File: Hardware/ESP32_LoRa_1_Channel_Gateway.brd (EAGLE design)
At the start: 25.4 x 45.7 mm, 84 parts, among them J3 USB, J4 QWIIC, J6 U.FL, Q1 MBT3904DW1T1, U1 3.3V, U2 CH340C, U3 ESP-WROOM-32NARROW, U4 RFM96W

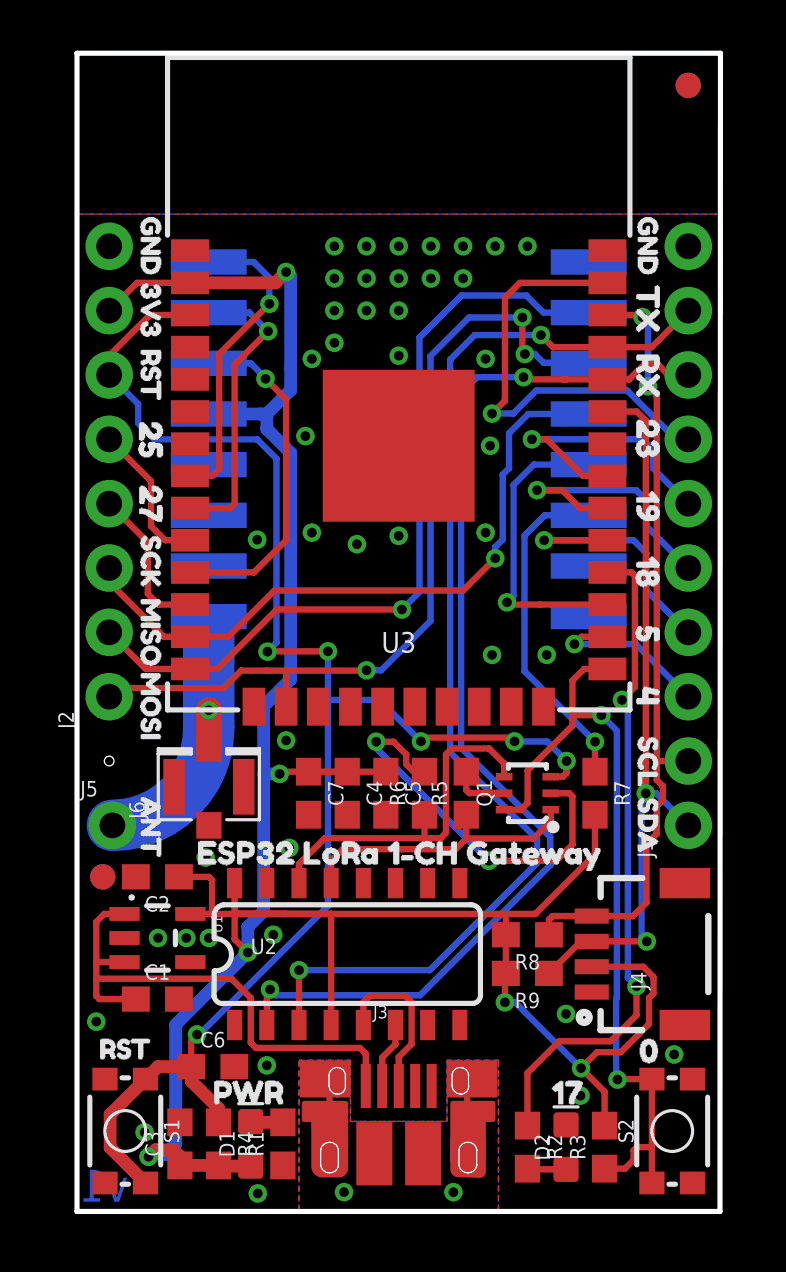
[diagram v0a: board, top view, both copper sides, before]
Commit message: Made changes from REDS review pt 1
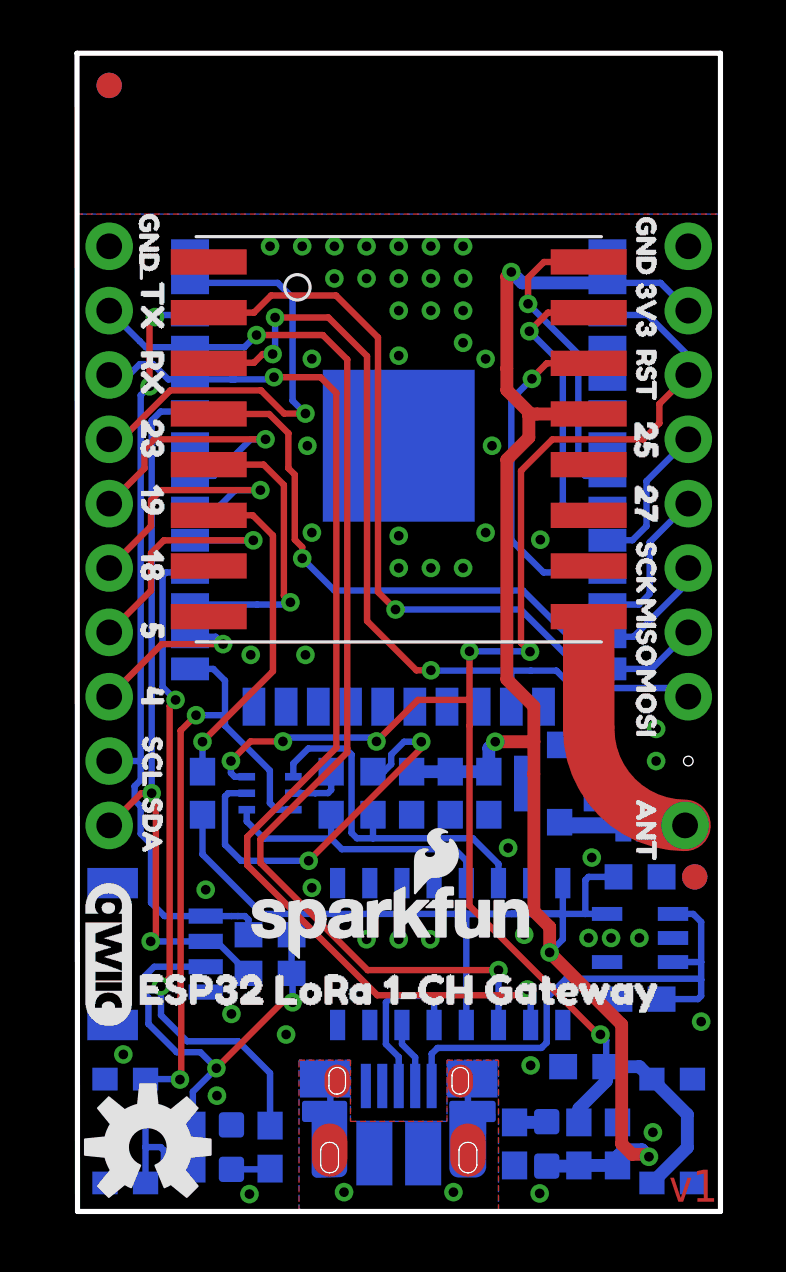
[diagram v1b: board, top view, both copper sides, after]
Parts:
- added JP1: JUMPER-SMT_2_NO_SILK, SparkFun-Jumpers:SMT-JUMPER_2_NO_SILK
- moved U$20 25.0 mm to (25.2, 6.41), flipped to the bottom
- moved FD3 23.4 mm to (24.4, 13.2), flipped to the bottom
- moved FD4 23.4 mm to (24.4, 13.2), flipped to the top
- moved U$9 23.0 mm to (25.9, 16.9), flipped to the bottom, turned to 0 degrees
- moved FD1 22.9 mm to (1.27, 44.5), flipped to the bottom
- moved FD2 22.9 mm to (1.27, 44.5), flipped to the top
- moved J1 22.9 mm to (1.27, 15.2), flipped to the bottom
- moved J2 22.9 mm to (24.1, 20.3), flipped to the bottom
- moved U$46 22.9 mm to (1.27, 10.2), flipped to the top
- moved J5 22.6 mm to (24.0, 15.2), flipped to the bottom
- moved U$45 22.6 mm to (1.40, 8.76), flipped to the top
- moved S1 21.6 mm to (23.5, 3.17), flipped to the bottom
- moved S2 21.6 mm to (1.91, 3.17), flipped to the bottom
- moved FRAME1 20.3 mm to (22.9, -7.62), flipped to the bottom
- moved LOGO1 19.8 mm to (2.79, 2.54), flipped to the top
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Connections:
- new net N$3: J6.FEED, JP1.1
- net ANT: now also JP1.2; no longer J6.FEED
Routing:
- net 3.3V: track 111.1 -> 115.4 mm
- net N$3: track 0.00 -> 2.57 mm
- net ANT: track 11.9 -> 12.1 mm, vias 1 -> 0

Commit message: Cosmetics
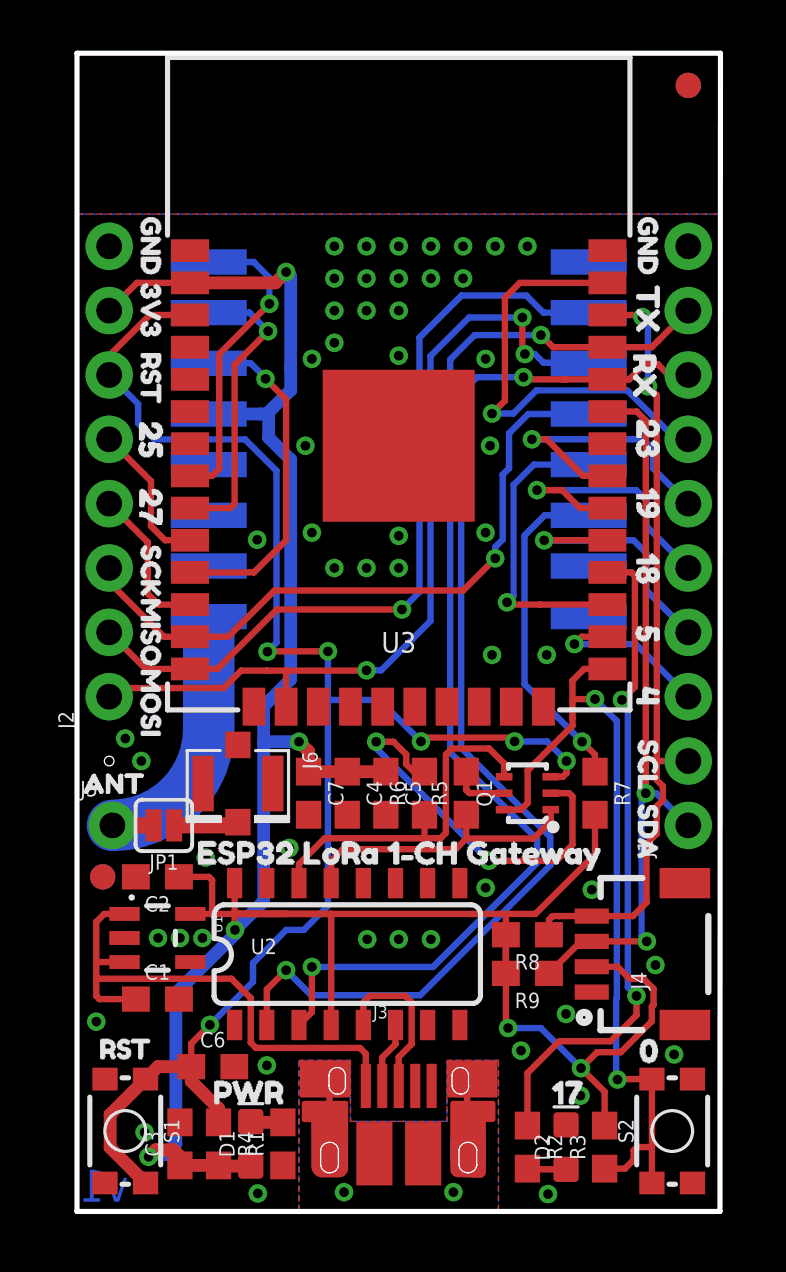
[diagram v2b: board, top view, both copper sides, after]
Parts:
- moved U$9 26.4 mm to (-0.48, 16.9), flipped to the top
- moved U$20 25.0 mm to (0.19, 6.41), flipped to the top
- moved FD3 23.4 mm to (1.02, 13.2), flipped to the top
- moved FD4 23.4 mm to (1.02, 13.2), flipped to the bottom
- moved FD1 22.9 mm to (24.1, 44.5), flipped to the top
- moved FD2 22.9 mm to (24.1, 44.5), flipped to the bottom
- moved J1 22.9 mm to (24.1, 15.2), flipped to the top
- moved J2 22.9 mm to (1.27, 20.3), flipped to the top
- moved U$46 22.9 mm to (24.1, 10.2), flipped to the bottom
- moved J5 22.6 mm to (1.40, 15.2), flipped to the top
- moved U$45 22.6 mm to (24.0, 8.76), flipped to the bottom
- moved S1 21.6 mm to (1.91, 3.17), flipped to the top
- moved S2 21.6 mm to (23.5, 3.17), flipped to the top
- moved FRAME1 20.3 mm to (2.54, -7.62), flipped to the top
- moved LOGO1 19.8 mm to (22.6, 2.54), flipped to the bottom
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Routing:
- net 3.3V: track 115.4 -> 116.2 mm
- net RXI: track 44.7 -> 45.4 mm
